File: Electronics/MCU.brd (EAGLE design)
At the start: 50 x 50 mm, 37 parts, among them IC2 74AC157D, J77 uart, U1 ATMEGA2560-16AU-TQFP100, U2 AT25DF041A-SH-B

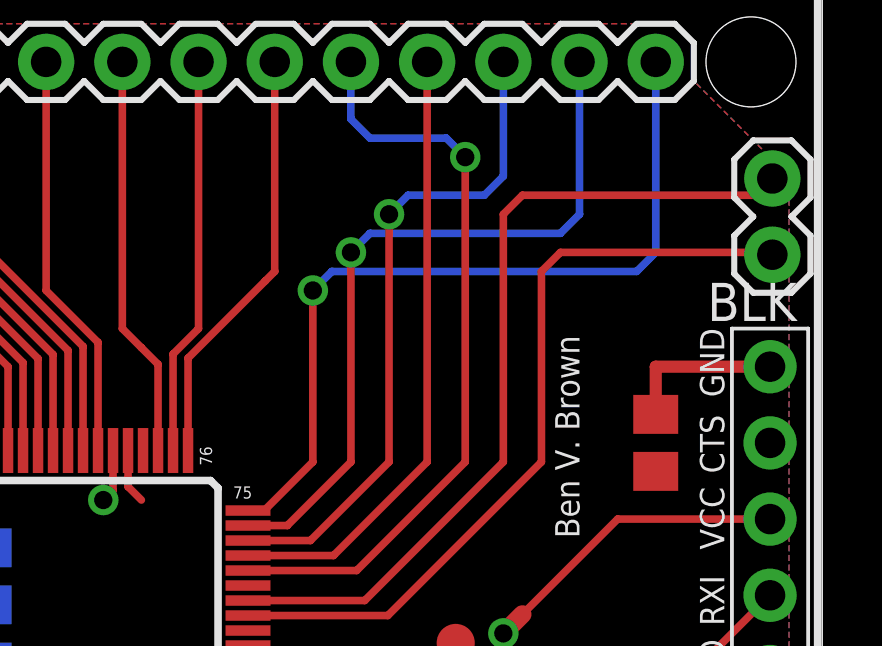
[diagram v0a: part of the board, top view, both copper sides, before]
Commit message: Gerbers!
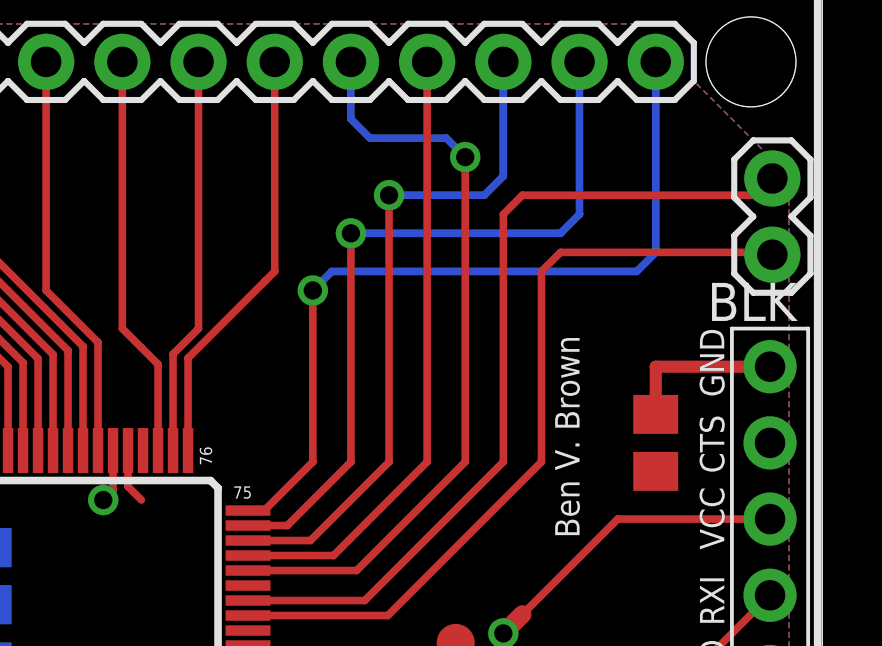
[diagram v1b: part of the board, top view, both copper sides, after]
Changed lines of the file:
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@@
 <wire x1="30.86" y1="31.67" x2="32.94" y2="31.67" width="0.254" layer="1"/>
 <wire x1="32.94" y1="31.67" x2="35.56" y2="34.29" width="0.254" layer="1"/>
-<wire x1="35.56" y1="34.29" x2="35.56" y2="42.545" width="0.254" layer="1"/>
-<via x="35.56" y="42.545" extent="1-16" drill="0.6096" shape="octagon"/>
-<wire x1="35.56" y1="42.545" x2="36.195" y2="43.18" width="0.254" layer="16"/>
-<wire x1="36.195" y1="43.18" x2="38.735" y2="43.18" width="0.254" layer="16"/>
+<wire x1="35.56" y1="34.29" x2="35.56" y2="43.18" width="0.254" layer="1"/>
+<via x="35.56" y="43.18" extent="1-16" drill="0.6096" shape="octagon"/>
+<wire x1="35.56" y1="43.18" x2="38.735" y2="43.18" width="0.254" layer="16"/>
 <wire x1="38.735" y1="43.18" x2="39.37" y2="43.815" width="0.254" layer="16"/>
 <wire x1="39.37" y1="43.815" x2="39.37" y2="47.625" width="0.254" layer="16"/>
@@
 <wire x1="30.86" y1="32.17" x2="32.17" y2="32.17" width="0.254" layer="1"/>
 <wire x1="32.17" y1="32.17" x2="34.29" y2="34.29" width="0.254" layer="1"/>
-<wire x1="34.29" y1="34.29" x2="34.29" y2="41.275" width="0.254" layer="1"/>
-<via x="34.29" y="41.275" extent="1-16" drill="0.6096" shape="octagon"/>
-<wire x1="34.29" y1="41.275" x2="34.925" y2="41.91" width="0.254" layer="16"/>
-<wire x1="34.925" y1="41.91" x2="41.275" y2="41.91" width="0.254" layer="16"/>
+<wire x1="34.29" y1="34.29" x2="34.29" y2="41.91" width="0.254" layer="1"/>
+<via x="34.29" y="41.91" extent="1-16" drill="0.6096" shape="octagon"/>
+<wire x1="34.29" y1="41.91" x2="41.275" y2="41.91" width="0.254" layer="16"/>
 <wire x1="41.275" y1="41.91" x2="41.91" y2="42.545" width="0.254" layer="16"/>
 <wire x1="41.91" y1="42.545" x2="41.91" y2="47.625" width="0.254" layer="16"/>
